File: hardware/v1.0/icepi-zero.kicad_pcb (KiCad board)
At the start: 4 copper layers, 65 x 30 mm, 138 parts, among them J1 Conn_02x20_Counter_Clockwise, J2 HDMI_C_1.3, J3 USB_C_Receptacle_USB2.0_14P, J4 USB_C_Receptacle_USB2.0_14P, J5 USB_C_Receptacle_USB2.0_14P, J6 Micro_SD_Card_Det2, SW1 SW_Push, U1 ECP5U_12_CABGA256, U10 W9825G6KH, U11 W25Q128JVS, U2 TLV62569DBV, U3 TLV62569DBV, U4 TLV62569DBV, U5 PCA9306DC1, U6 FT231XQ, U7 TPD2EUSB30A, U8 TPD2EUSB30A, U9 TPD2EUSB30A, Y1 SITxxxxxx-1x-33E-50.000000

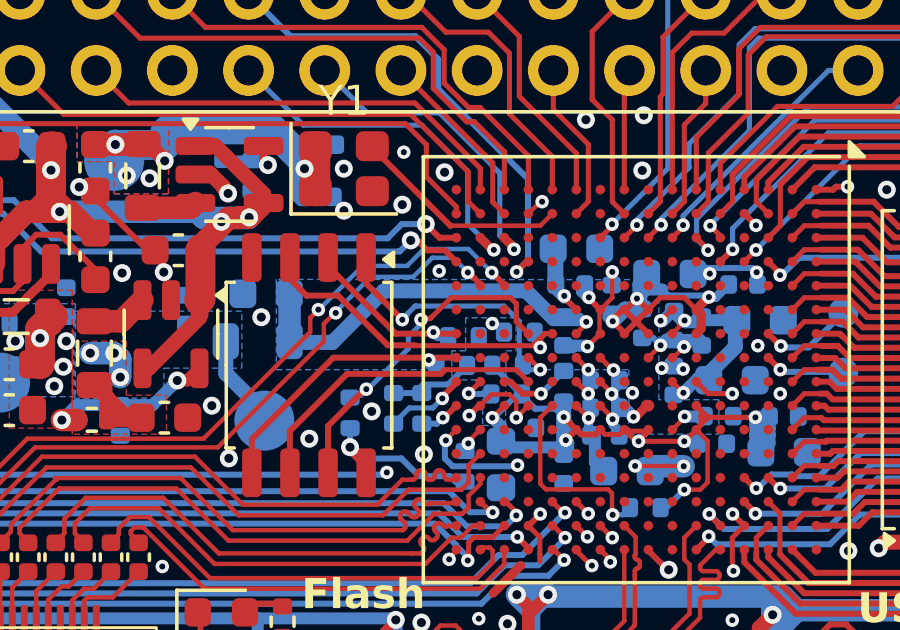
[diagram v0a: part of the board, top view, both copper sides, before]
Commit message: Forgot to commit yesterday
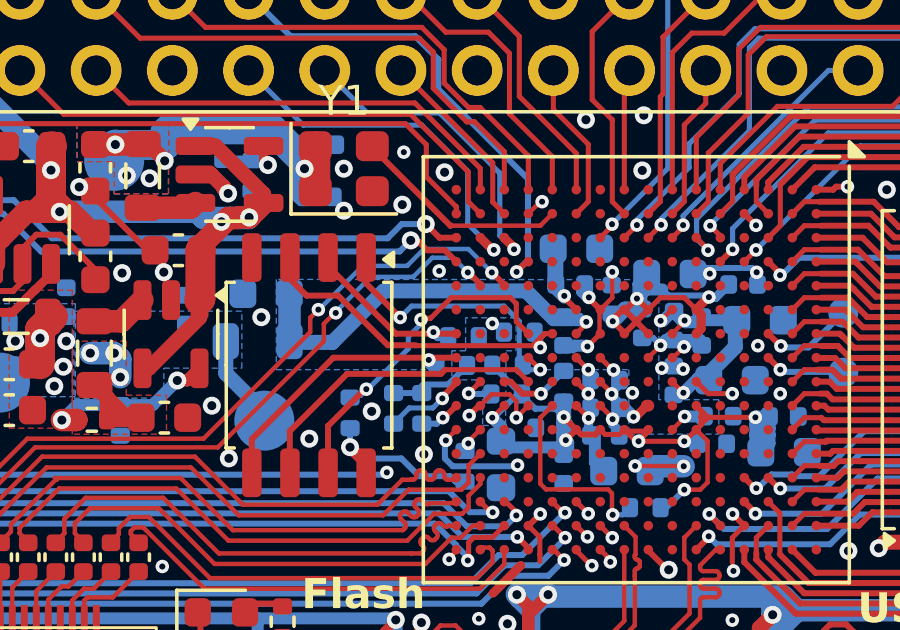
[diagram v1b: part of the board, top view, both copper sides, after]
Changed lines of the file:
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@@
 	)
 	(segment
-		(start 142.148768 103.008768)
-		(end 142.2 103.06)
+		(start 140.995 101.875)
+		(end 140.995 101.2125)
 		(width 0.2)
 		(layer "F.Cu")
@@
 	)
 	(segment
-		(start 142.2 103.085)
-		(end 142.13 103.015)
-		(width 0.2)
-		(layer "F.Cu")
-		(net 23)
-	)
-	(segment
-		(start 142.13 103.015)
-		(end 142.13 103.01)
-		(width 0.2)
-		(layer "F.Cu")
-		(net 23)
-	)
-	(segment
-		(start 140.995 101.875)
-		(end 140.995 101.2125)
+		(start 142.13 103.01)
+		(end 140.995 101.875)
 		(width 0.2)
 		(layer "F.Cu")
@@
 	(segment
 		(start 142.13 103.01)
-		(end 140.995 101.875)
+		(end 142.131232 103.008768)
 		(width 0.2)
 		(layer "F.Cu")
@@
 	)
 	(segment
-		(start 142.2 103.06)
-		(end 142.2 103.085)
+		(start 142.131232 103.008768)
+		(end 142.148768 103.008768)
 		(width 0.2)
 		(layer "F.Cu")
@@
 	)
 	(via
-		(at 142.2 103.085)
+		(at 142.13 103.01)
 		(size 0.45)
 		(drill 0.2)
 		(layers "F.Cu" "B.Cu")
-		(net 23)
-	)
-	(segment
-		(start 142.358385 102.898189)
-		(end 142.622574 102.634)
-		(width 0.17)
-		(layer "B.Cu")
 		(net 23)
 	)
@@
 	)
 	(segment
-		(start 142.655 102.63)
-		(end 145.59 102.63)
+		(start 146.1 103.14)
+		(end 146.1 104.48)
 		(width 0.17)
 		(layer "B.Cu")
@@
 	)
 	(segment
-		(start 146.1 103.14)
-		(end 146.1 104.48)
+		(start 145.59 102.63)
+		(end 146.1 103.14)
 		(width 0.17)
 		(layer "B.Cu")
@@
 	)
 	(segment
-		(start 142.651 102.634)
-		(end 142.655 102.63)
+		(start 142.13 103.01)
+		(end 142.51 102.63)
 		(width 0.17)
 		(layer "B.Cu")
@@
 	)
 	(segment
-		(start 142.622574 102.634)
-		(end 142.651 102.634)
-		(width 0.17)
-		(layer "B.Cu")
-		(net 23)
-	)
-	(segment
-		(start 142.2 103.085)
-		(end 142.358385 102.926615)
-		(width 0.17)
-		(layer "B.Cu")
-		(net 23)
-	)
-	(segment
-		(start 145.59 102.63)
-		(end 146.1 103.14)
-		(width 0.17)
-		(layer "B.Cu")
-		(net 23)
-	)
-	(segment
-		(start 142.358385 102.926615)
-		(end 142.358385 102.898189)
+		(start 142.51 102.63)
+		(end 145.59 102.63)
 		(width 0.17)
 		(layer "B.Cu")
@@
 	)
 	(segment
-		(start 139.725 101.295)
-		(end 139.725 101.0125)
+		(start 144 103.55)
+		(end 141.98 103.55)
 		(width 0.2)
 		(layer "F.Cu")
@@
 	)
 	(segment
-		(start 144 103.55)
-		(end 141.98 103.55)
+		(start 139.725 101.295)
+		(end 139.725 101.0125)
 		(width 0.2)
 		(layer "F.Cu")

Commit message: Finish lpf
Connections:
- net FPDI_CEC renamed GPDI_CEC
- net FPDI_CLK+ renamed GPDI_CLK+
- net FPDI_CLK- renamed GPDI_CLK-
- net FPDI_D0+ renamed GPDI_D0+
- net FPDI_D0- renamed GPDI_D0-
- net FPDI_D1+ renamed GPDI_D1+
- net FPDI_D1- renamed GPDI_D1-
- net FPDI_D2+ renamed GPDI_D2+
- net FPDI_D2- renamed GPDI_D2-
- net FPDI_HPD renamed GPDI_HPD
- net FPDI_UTIL renamed GPDI_UTIL
- net Net-(J2-CEC) renamed /GPIO/CONN_CEC
- net Net-(J2-HPD) renamed /GPIO/CONN_HPD
- net Net-(J2-UTILITY) renamed /GPIO/CONN_UTIL
- J2 pad 15: GPDI_SCL -> /GPIO/GPDI_SCK
- R18 pad 2: FPDI_SDA -> GPDI_SDA
- R19 pad 2: FPDI_SCL -> /GPIO/GPDI_SCK
- U1 pad T3: FPDI_SCL -> GPDI_SCL
- U1 pad T4: FPDI_SDA -> GPDI_SDA
- U5 pad 3: FPDI_SCL -> /GPIO/GPDI_SCK
- U5 pad 4: FPDI_SDA -> GPDI_SDA
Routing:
- net GPDI_SDA: track 7.01 -> 44.9 mm, vias 0 -> 2
- net FPDI_SDA: track 37.9 -> 0.00 mm, vias 2 -> 0
- net GPDI_SCL: track 10.5 -> 48.2 mm, vias 2 -> 4
- net FPDI_SCL: track 37.6 -> 0.00 mm, vias 2 -> 0
